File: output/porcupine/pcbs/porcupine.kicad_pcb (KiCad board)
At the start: 2 copper layers, 129.4 x 113.9 mm, 54 parts, among them J1 Jumper, J2 Jumper

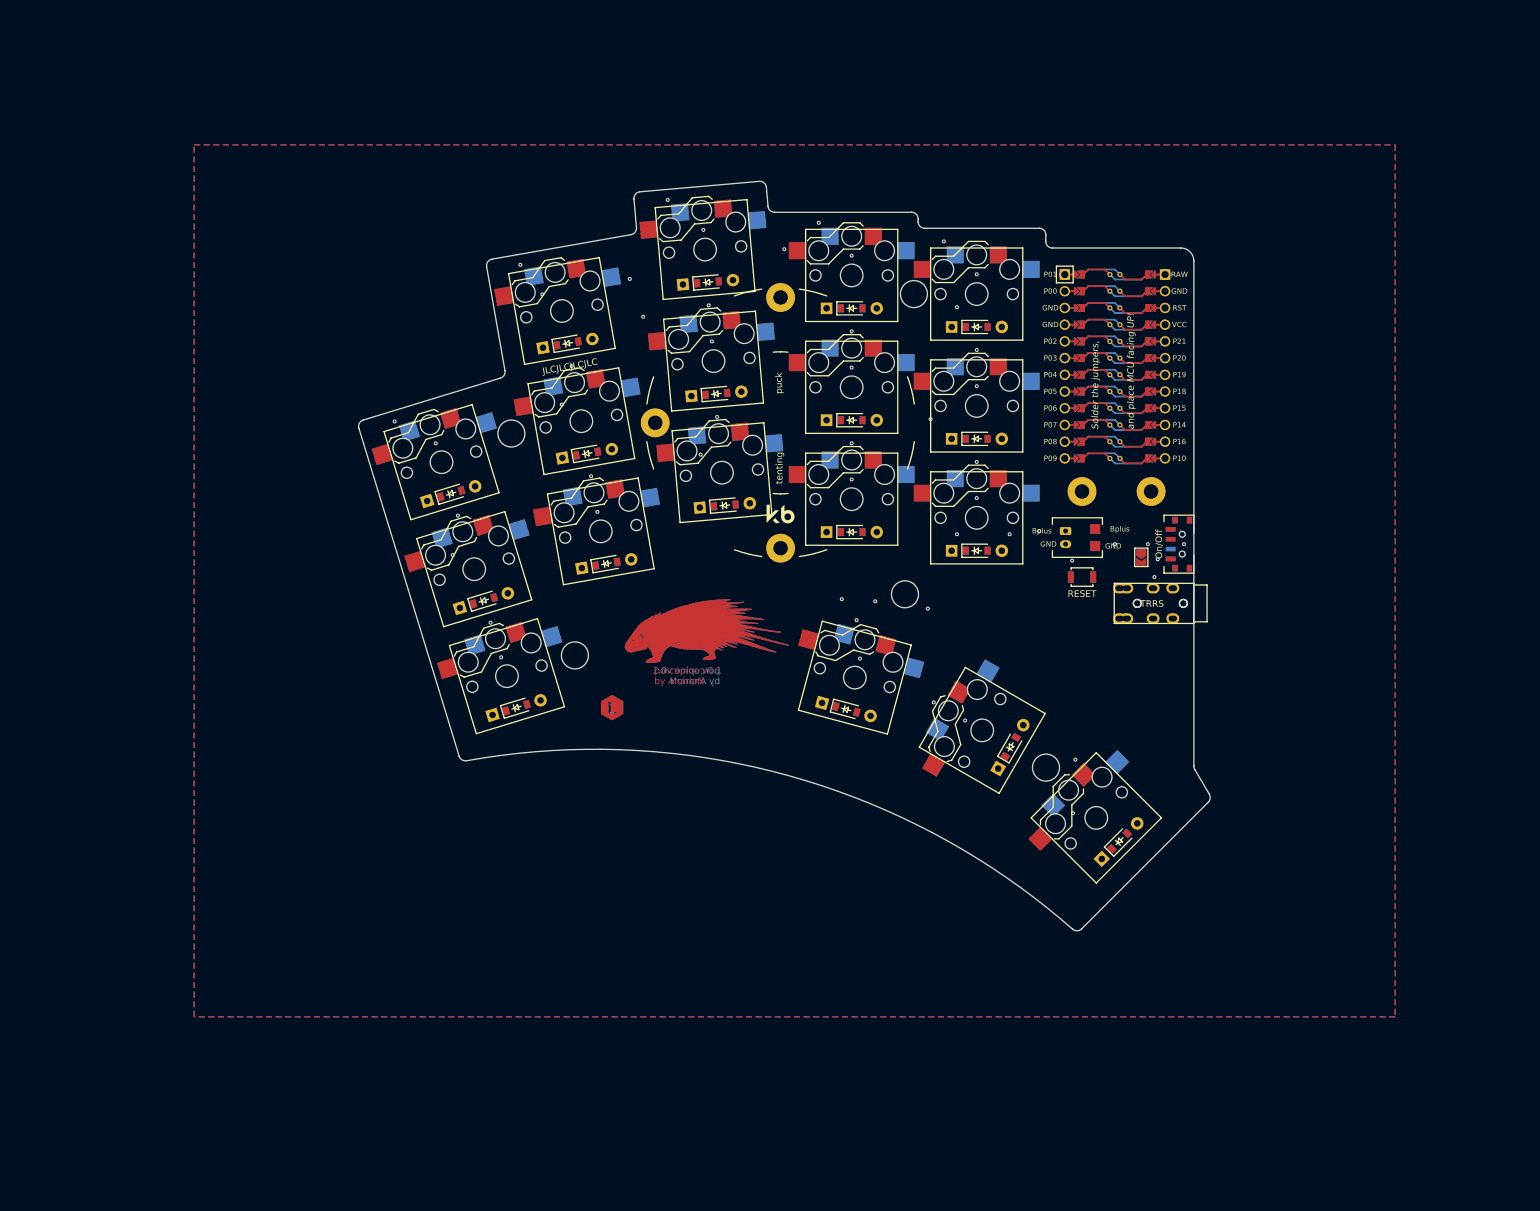
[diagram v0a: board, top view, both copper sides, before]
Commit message: 🔥 Remove old versions
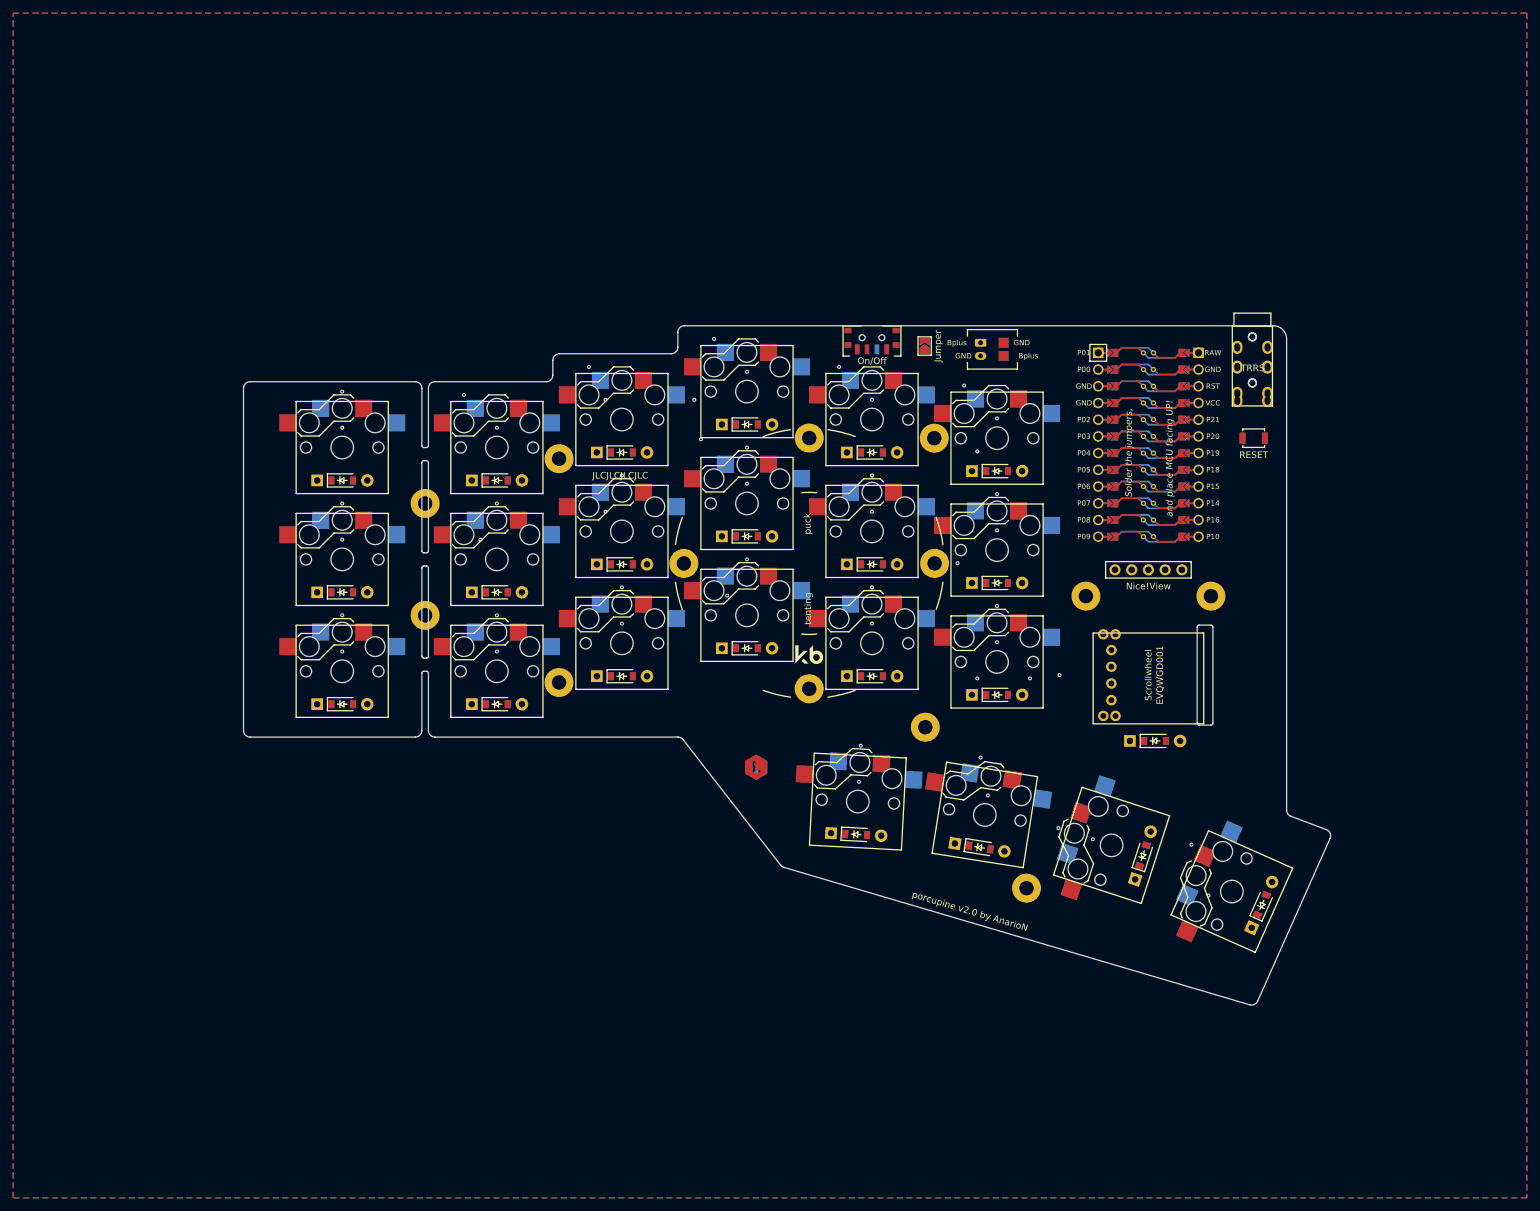
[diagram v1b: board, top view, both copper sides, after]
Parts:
- removed LOGO_B, LOGO_F: , Porcupine Logo
- removed _9: Tenting Puck, Tenting Puck
- added D19: D_SOD-123, Diode_SMD:SOD-123, F.Cu at (228.1, 174.8)
- added D20: D_SOD-123, Diode_SMD:SOD-123, F.Cu at (246.9, 176.8)
- added D21: D_SOD-123, Diode_SMD:SOD-123, F.Cu at (271.7, 178.0)
- added D22: D_SOD-123, Diode_SMD:SOD-123, F.Cu at (289.8, 185.5)
- added D23: D_SOD-123, Diode_SMD:SOD-123, F.Cu at (273.5, 160.6)
- added Nice!View1: , lib:niceview_headers, F.Cu at (272.5, 134.6)
- added REF**: RollerEncoder_Panasonic_EVQWGD001, RollerEncoder_Panasonic_EVQWGD001, F.Cu at (272.5, 150.6)
- added S19: , PG1350, F.Cu at (228.3, 169.8)
- added S20: , PG1350, F.Cu at (247.6, 171.8)
- added S21: , PG1350, F.Cu at (266.9, 176.5)
- added S22: , PG1350, F.Cu at (285.2, 183.5)
- added _67: hole, Through Hole, F.Cu at (263.0, 138.6)
- added _68: hole, Through Hole, F.Cu at (282.0, 138.6)
- added _69: hole, Through Hole, F.Cu at (162.6, 124.5)
- added _7: Tenting Puck, Tenting Puck, F.Cu at (221.0, 133.6)
- added _70: hole, Through Hole, F.Cu at (162.6, 141.5)
- added _71: hole, Through Hole, F.Cu at (182.9, 117.7)
- added _72: hole, Through Hole, F.Cu at (182.9, 151.7)
- added _75: hole, Through Hole, F.Cu at (254.0, 183.0)
- moved S18 59.6 mm to (249.5, 114.6), turned to 0 degrees
- moved D18 59.2 mm to (249.5, 119.6), turned to 0 degrees
- moved _3 56.2 mm to (230.5, 99.7), turned to 180 degrees
- moved _74 49.6 mm to (238.6, 158.5)
- moved J1 46.0 mm to (238.5, 100.6), turned to 90 degrees
- moved J2 46.0 mm to (238.5, 100.6), turned to 90 degrees
- moved TRRS_B 43.0 mm to (288.3, 97.6), turned to 0 degrees
- moved TRRS_F 43.0 mm to (288.3, 97.6), turned to 0 degrees
- moved PAD2 33.9 mm to (250.5, 100.1)
- moved _4_B 33.6 mm to (288.5, 114.6)
- moved _4_F 33.6 mm to (288.5, 114.6)
- moved _2 31.4 mm to (247.0, 101.1)
- moved D7 30.3 mm to (192.5, 150.8), turned to 0 degrees
- moved S7 30.1 mm to (192.5, 145.8), turned to 0 degrees
- moved PAD1 29.8 mm to (250.5, 102.1)
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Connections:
- net P0 renamed trrs
- D1 pad 1: pinky_bottom -> outer_bottom
- D1 pad 2: P6 -> outer_bottom
- D10 pad 1: index_bottom -> middle_bottom
- D10 pad 2: P6 -> middle_bottom
- D11 pad 1: index_home -> middle_home
- D11 pad 2: P5 -> middle_home
- D12 pad 1: index_top -> middle_top
- D12 pad 2: P4 -> middle_top
- D13 pad 1: inner_bottom -> index_bottom
- D13 pad 2: P6 -> index_bottom
- D14 pad 1: inner_home -> index_home
- D14 pad 2: P5 -> index_home
- D15 pad 1: inner_top -> index_top
- D15 pad 2: P4 -> index_top
- D16 pad 1: near_thumb -> inner_bottom
- D16 pad 2: P7 -> inner_bottom
- D17 pad 1: home_thumb -> inner_home
- D17 pad 2: P7 -> inner_home
- D18 pad 1: far_thumb -> inner_top
- D18 pad 2: P7 -> inner_top
- D2 pad 1: pinky_home -> outer_home
- D2 pad 2: P5 -> outer_home
- D3 pad 1: pinky_top -> outer_top
- D3 pad 2: P4 -> outer_top
- D4 pad 1: ring_bottom -> pinky_bottom
- D4 pad 2: P6 -> pinky_bottom
- D5 pad 1: ring_home -> pinky_home
- D5 pad 2: P5 -> pinky_home
- D6 pad 1: ring_top -> pinky_top
- D6 pad 2: P4 -> pinky_top
- D7 pad 1: middle_bottom -> ring_bottom
- D7 pad 2: P6 -> ring_bottom
- D8 pad 1: middle_home -> ring_home
- D8 pad 2: P5 -> ring_home
- D9 pad 1: middle_top -> ring_top
- D9 pad 2: P4 -> ring_top
- MCU1 pad 10: P14 -> col_middle
- MCU1 pad 11: P16 -> col_index
- MCU1 pad 12: P10 -> col_inner
- MCU1 pad 15: P7 -> row_thumb
- MCU1 pad 16: P6 -> row_bottom
- MCU1 pad 17: P5 -> row_home
- MCU1 pad 18: P4 -> row_top
- MCU1 pad 19: P3 -> SCL
- MCU1 pad 20: P2 -> SDA
- MCU1 pad 24: P1 -> CS
- MCU1 pad 5: P21 -> ENCB
- MCU1 pad 6: P20 -> ENCA
- MCU1 pad 7: P19 -> col_outer
- MCU1 pad 8: P18 -> col_pinky
- MCU1 pad 9: P15 -> col_ring
- S1 pad 1: pinky_bottom -> outer_bottom
- S1 pad 2: P20 -> col_outer
- S10 pad 1: index_bottom -> middle_bottom
- S10 pad 2: P15 -> col_middle
- S11 pad 1: index_home -> middle_home
- S11 pad 2: P15 -> col_middle
- S12 pad 1: index_top -> middle_top
- S12 pad 2: P15 -> col_middle
- S13 pad 1: inner_bottom -> index_bottom
- S13 pad 2: P14 -> col_index
- S14 pad 1: inner_home -> index_home
- S14 pad 2: P14 -> col_index
- S15 pad 1: inner_top -> index_top
- S15 pad 2: P14 -> col_index
- S16 pad 1: near_thumb -> inner_bottom
- S16 pad 2: P18 -> col_inner
- S17 pad 1: home_thumb -> inner_home
- S17 pad 2: P15 -> col_inner
- S18 pad 1: far_thumb -> inner_top
- S18 pad 2: P14 -> col_inner
- S2 pad 1: pinky_home -> outer_home
- S2 pad 2: P20 -> col_outer
- S3 pad 1: pinky_top -> outer_top
- S3 pad 2: P20 -> col_outer
- S4 pad 1: ring_bottom -> pinky_bottom
- S4 pad 2: P19 -> col_pinky
- S5 pad 1: ring_home -> pinky_home
- S5 pad 2: P19 -> col_pinky
- S6 pad 1: ring_top -> pinky_top
- S6 pad 2: P19 -> col_pinky
- S7 pad 1: middle_bottom -> ring_bottom
- S7 pad 2: P18 -> col_ring
- S8 pad 1: middle_home -> ring_home
- S8 pad 2: P18 -> col_ring
- S9 pad 1: middle_top -> ring_top
- S9 pad 2: P18 -> col_ring
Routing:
- net outer_top: vias 0 -> 1
- net outer_home: vias 0 -> 1
- net outer_bottom: vias 0 -> 1
- net inner_thumb: vias 0 -> 1
- net col_ring: vias 0 -> 4
- net col_pinky: vias 0 -> 3
- net col_outer: vias 0 -> 3
- net col_middle: vias 0 -> 4
- net col_inner: vias 0 -> 4
- net col_index: vias 0 -> 4
- net RST: vias 2 -> 0
- net RAW: vias 1 -> 0
- net P20: vias 3 -> 0
- net P19: vias 3 -> 0
- net P18: vias 5 -> 0
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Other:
- board size 129.4 x 113.9 mm -> 165.2 x 103.2 mm
- net class Default removed
- net class Power removed
- board text added: "porcupine v2.0 by AnarioN"
- board text removed: "porcupine v0.1 by AnarioN"
